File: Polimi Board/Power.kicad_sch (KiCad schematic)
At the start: 7 parts, among them J4 Jack-DC, U5 MCP1826S, U6 MCP1826S

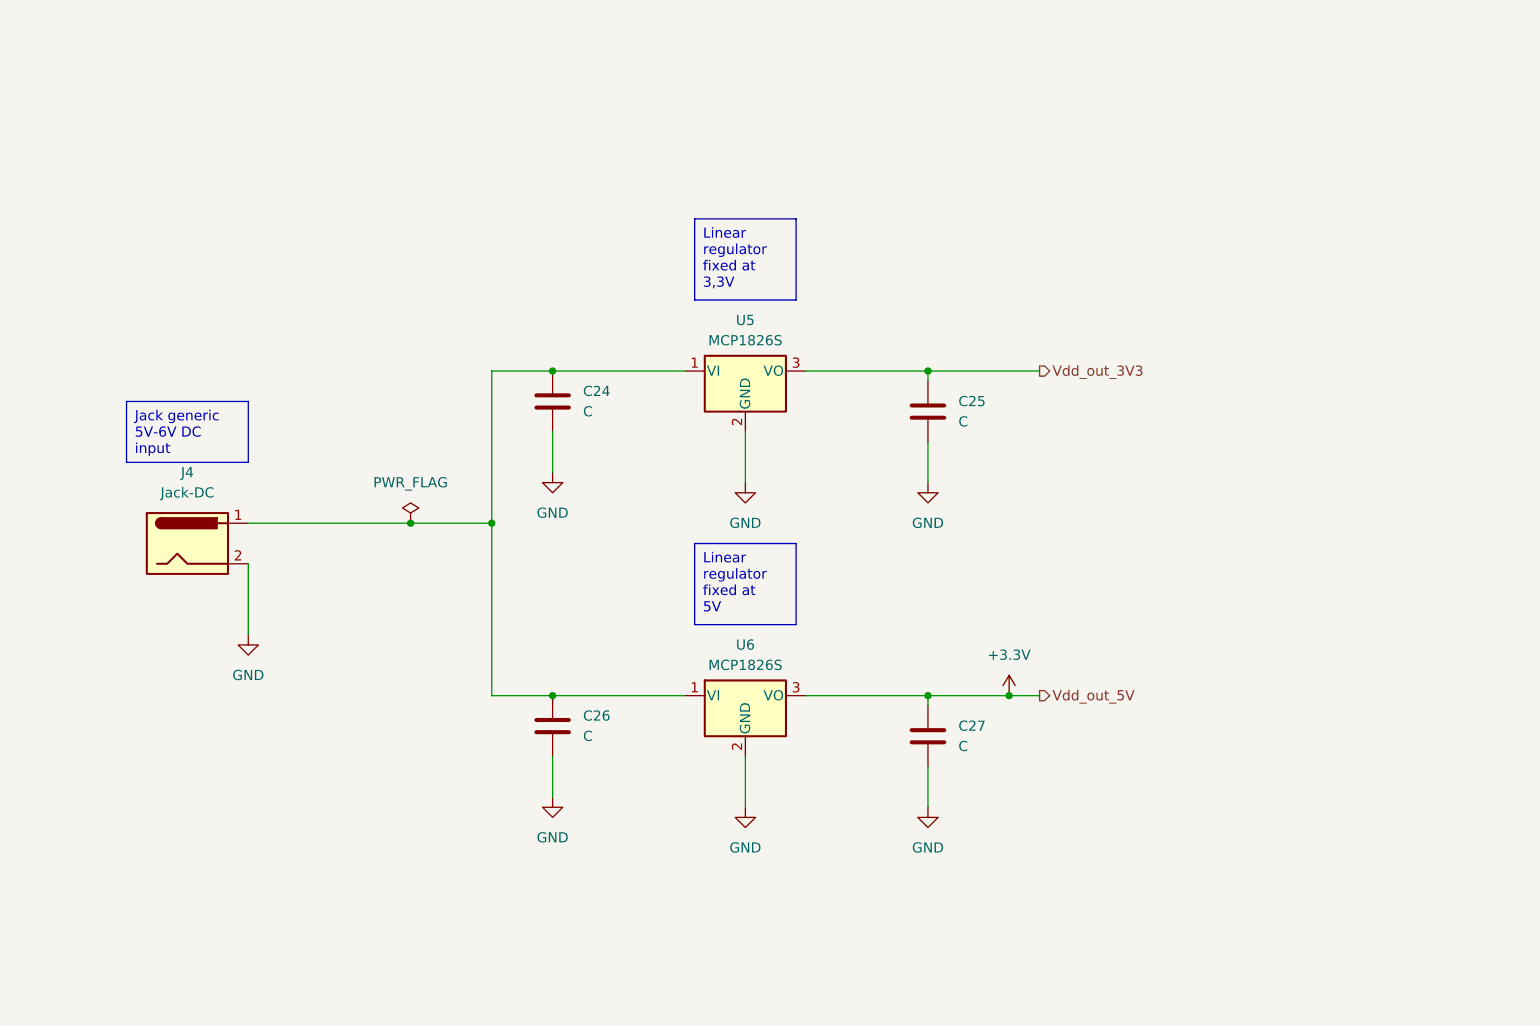
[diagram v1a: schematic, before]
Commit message: Update the design with new specifications
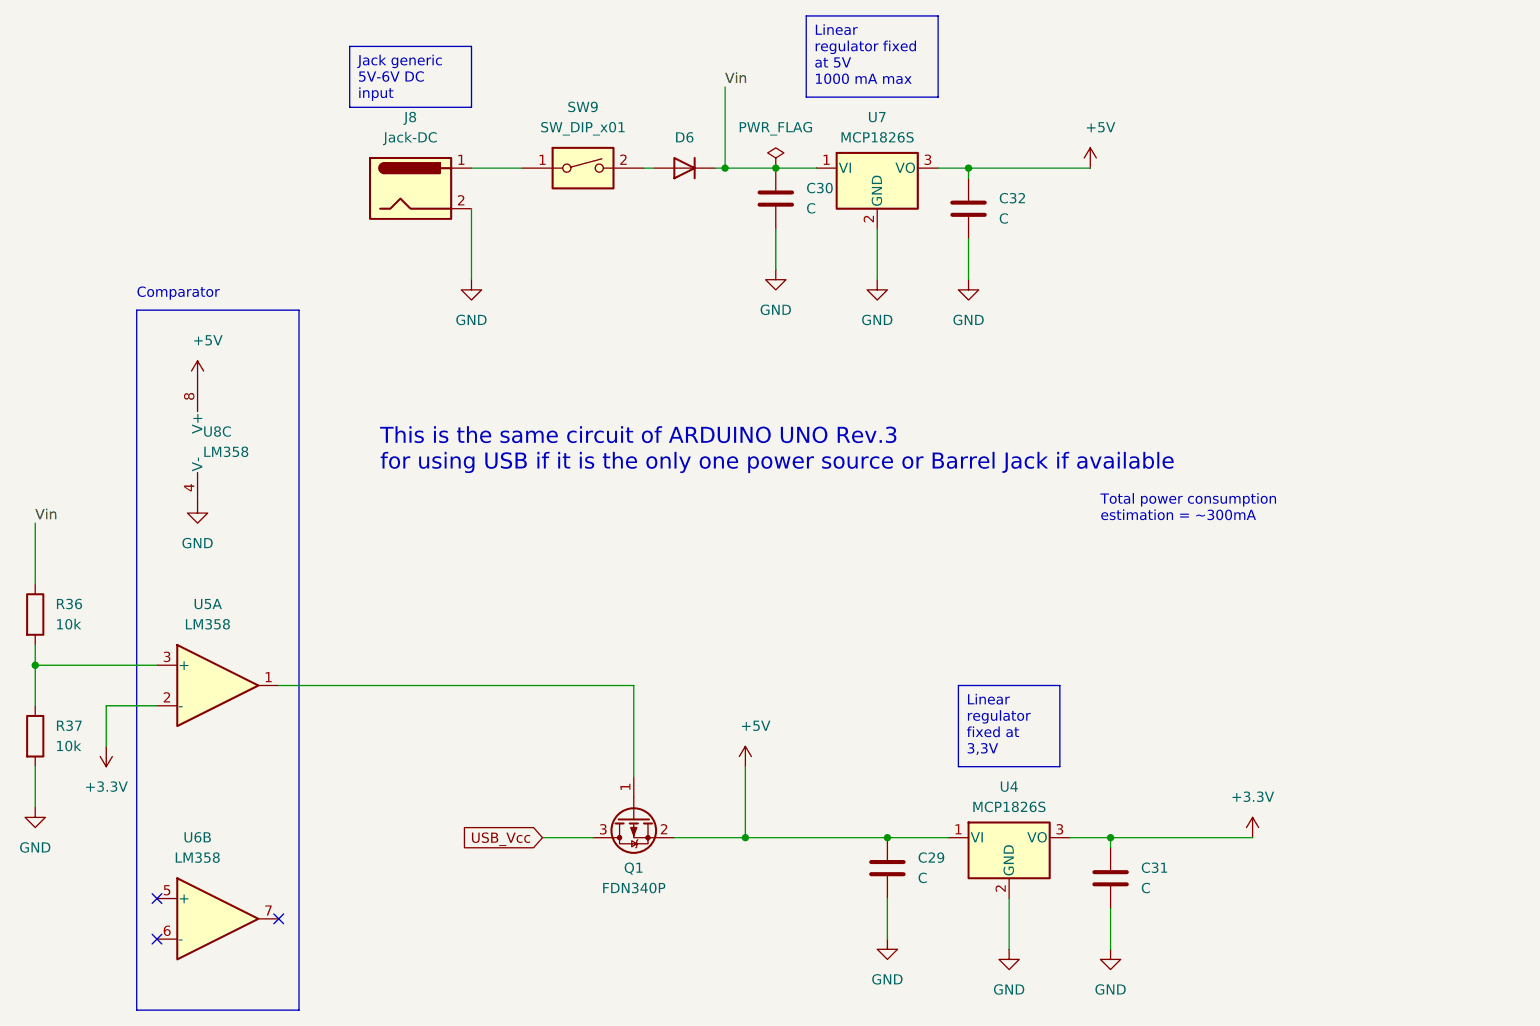
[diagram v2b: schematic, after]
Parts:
- removed C24, C25, C26, C27: C, symbol Device:C
- removed J4: Jack-DC, Connector_BarrelJack:BarrelJack_SwitchcraftConxall_RAPC10U_Horizontal, symbol Connector:Jack-DC
- removed U5, U6: MCP1826S, Package_TO_SOT_SMD:SOT-223-3_TabPin2, symbol Regulator_Linear:MCP1826S
- added C29, C30, C31, C32: C, symbol Device:C
- added D6: ~, symbol Device:D
- added J8: Jack-DC, Connector_BarrelJack:BarrelJack_SwitchcraftConxall_RAPC10U_Horizontal, symbol Connector:Jack-DC
- added Q1: FDN340P, Package_TO_SOT_SMD:SOT-23, symbol Transistor_FET:FDN340P
- added R36, R37: 10k, symbol Device:R
- added SW9: SW_DIP_x01, symbol Switch:SW_DIP_x01
- added U4, U7: MCP1826S, Package_TO_SOT_SMD:SOT-223-3_TabPin2, symbol Regulator_Linear:MCP1826S
- added U5, U6, U8: LM358, symbol Amplifier_Operational:LM358
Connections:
- net +3.3V: now also C31.1, U4.3 (VO), U5.2 (-)
- net GND: now also C29.2, C30.2, C31.2, C32.2, J8.2, R37.2, U4.2 (GND), U7.2 (GND), U8.4 (V-)
- new net: D6.2 (A), SW9.2
- new net: J8.1, SW9.1
- new net: Q1.1 (G), U5.1
- new net: R36.2, R37.1, U5.3 (+)
- new net +5V: C29.1, C32.1, Q1.2 (S), U4.1 (VI), U7.3 (VO), U8.8 (V+)
- new net USB_Vcc: Q1.3 (D)
- new net Vin: C30.1, D6.1 (K), R36.1, U7.1 (VI)
- no-connect marks 0 -> 3
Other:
- note added: "Comparator"
- note added: "This is the same circuit of ARDUINO UNO Rev.3 for using USB if it is the only one power source or Barrel Jack if available"
- note added: "Total power consumption estimation = ~300mA"
